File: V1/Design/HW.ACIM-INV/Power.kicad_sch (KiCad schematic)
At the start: 106 parts, among them J1 AC POWER INPUT, J2 FAN, M4 470V/1.2kA, M5 470V/1.2kA, M6 470V/1.2kA, M7 470V/1.2kA, Q10 20V/1A, Q11 20V/1A, U10 SMPS 12V±2%/0.8A, U13 LDO 3.3V±0.5%/1A, U14 SMPS 15V±2%/0.6A, U17 LDO 5V±0.4%/250mA, U20 SMPS 5V±2%/1.2A

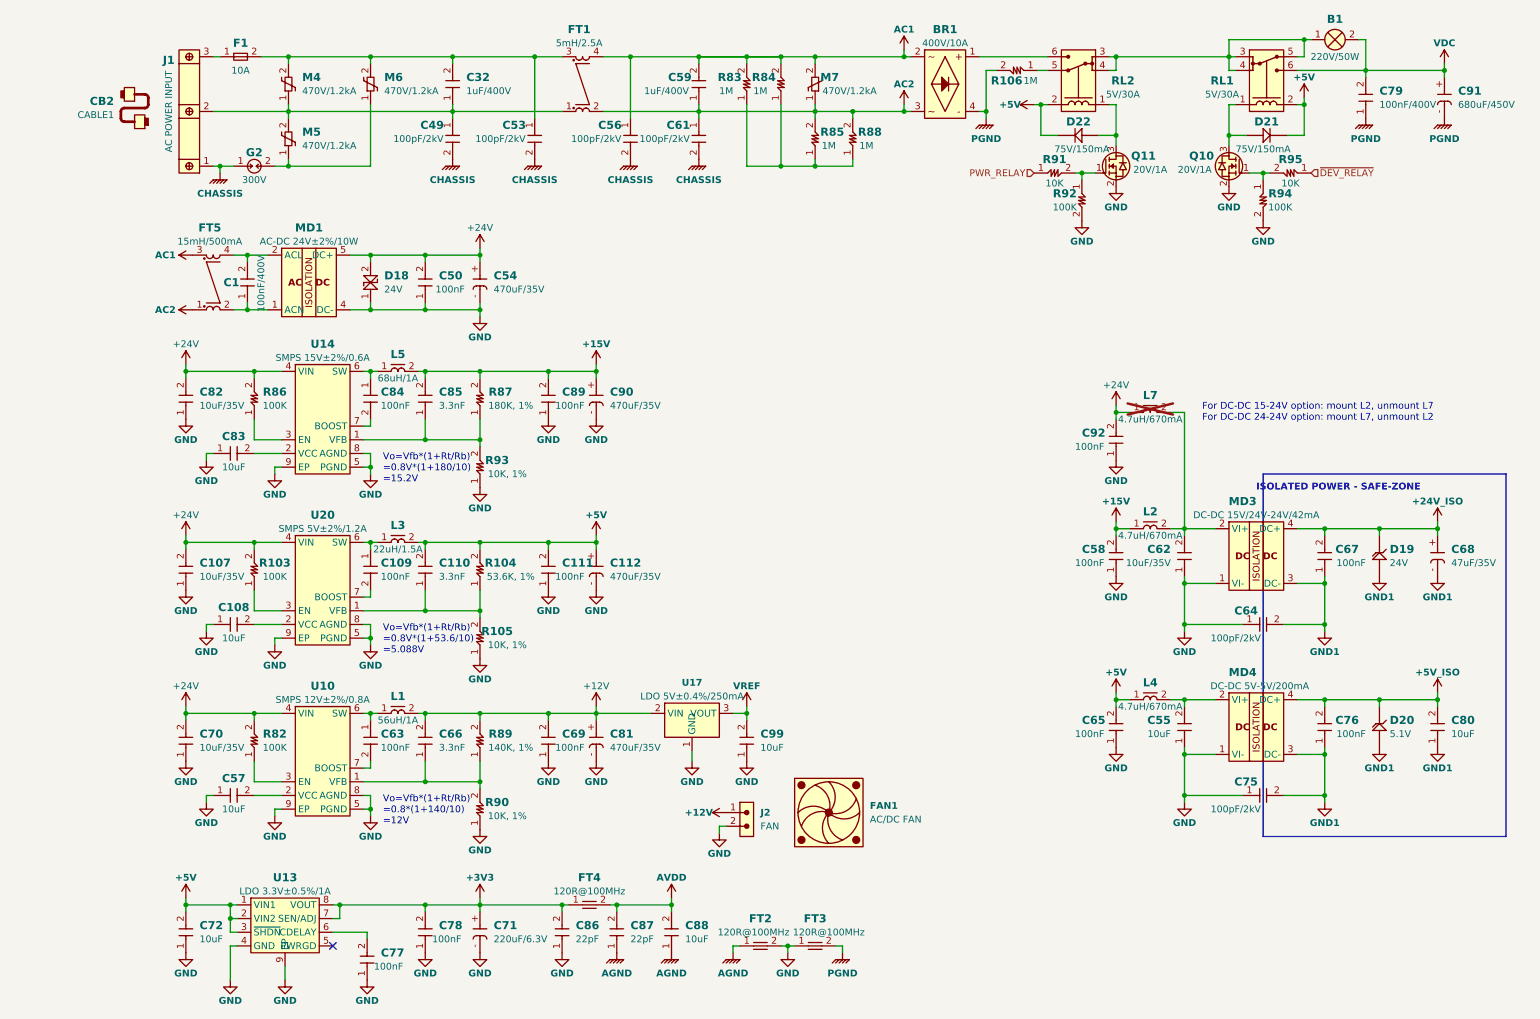
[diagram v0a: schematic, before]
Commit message: V1 schematic update 11
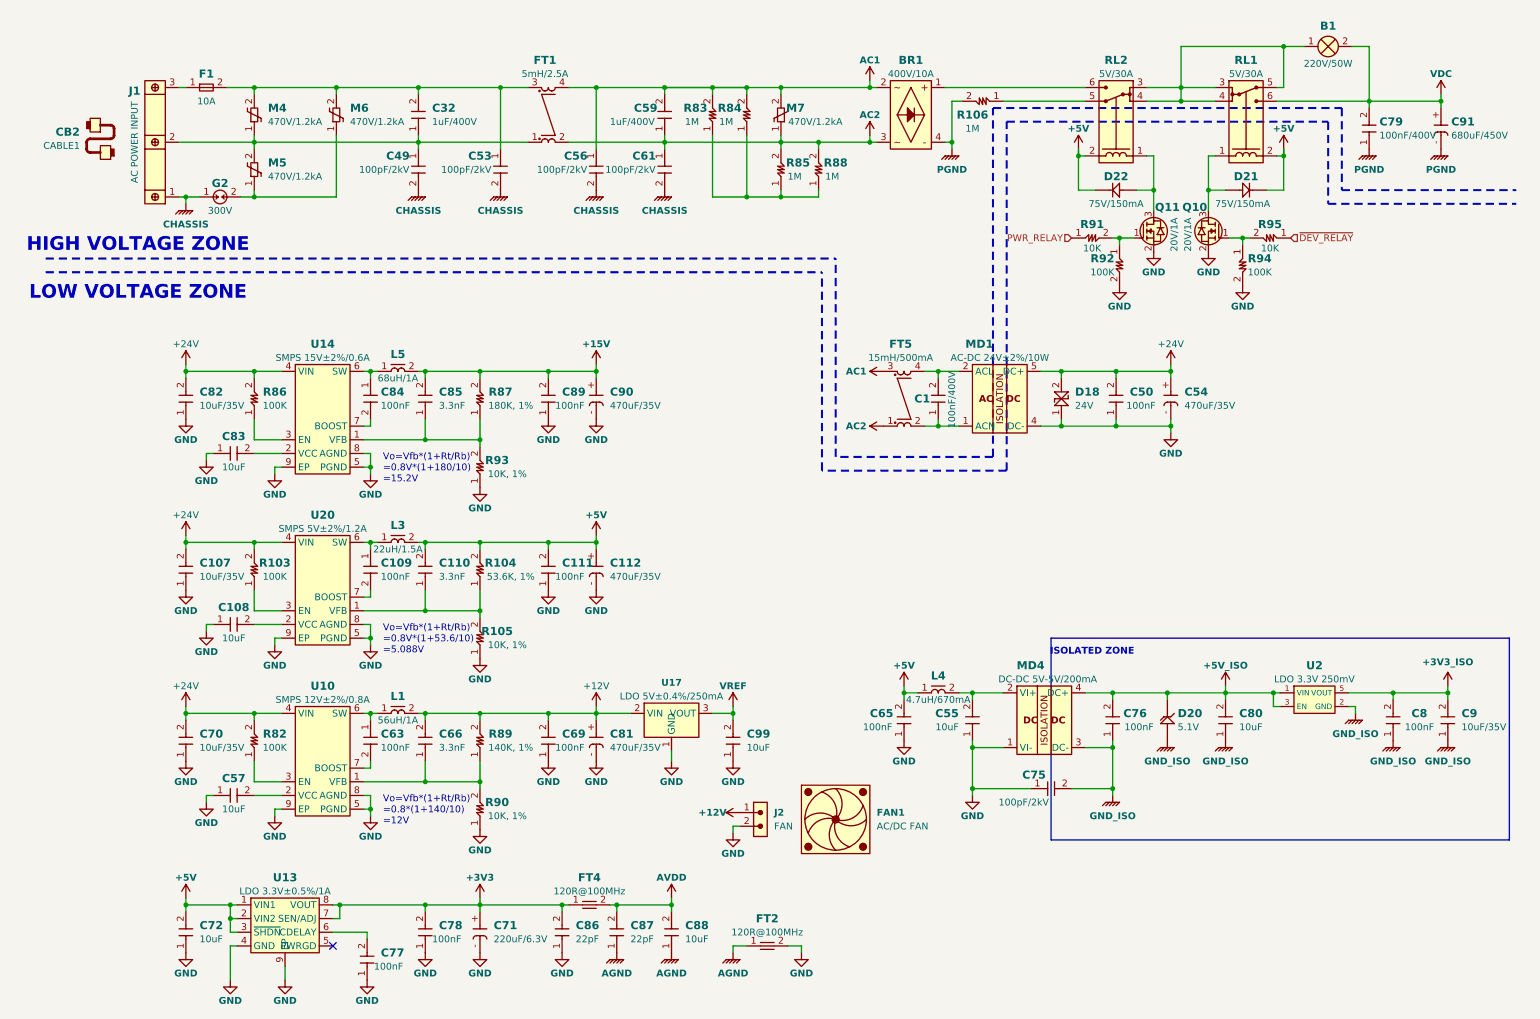
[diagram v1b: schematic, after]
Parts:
- removed C58, C67, C92: 100nF, SAMPI:CAP0603, symbol SAMPI:CERCAP
- removed C62: 10uF/35V, SAMPI:CAP0603, symbol SAMPI:CERCAP
- removed C64: 100pF/2kV, SAMPI:CAP1206, symbol SAMPI:CERCAP
- removed C68: 47uF/35V, SAMPI:CAP_ELEC-6.6x6.6-DIA6.3, symbol SAMPI:ELECCAP
- removed D19: 24V, SAMPI:SOD-80C_DO-213AC, symbol SAMPI:DIODE-ZEN
- removed FT3: 120R@100MHz, SAMPI:FT0603, symbol SAMPI:FerriteBead
- removed L2, L7: 4.7uH/670mA, SAMPI:IND-R5-2MM-TH, symbol SAMPI:IND
- removed MD3: DC-DC 15V/24V-24V/42mA, SAMPI:B1524S-1WR3, symbol SAMPI:DC-DC
- added C8: 100nF, SAMPI:CAP0603, symbol SAMPI:CERCAP
- added C9: 10uF/35V, SAMPI:CAP0603, symbol SAMPI:CERCAP
- added U2: LDO 3.3V 250mV, symbol SAMPI:MIC5504_2
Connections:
- net +5V_ISO: now also U2.1 (VIN), U2.3 (EN)
- net GND1 renamed GND_ISO
- net GND_ISO: now also C8.1, C9.1, U2.2 (GND)
- new net +3V3_ISO: C8.2, C9.2, U2.5 (VOUT)
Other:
- note added: "HIGH VOLTAGE ZONE"
- note added: "ISOLATED ZONE"
- note added: "LOW VOLTAGE ZONE"
- note removed: "For DC-DC 15-24V option: mount L2, unmount L7 For DC-DC 24-24V option: mount L7, unmount L2"
- note removed: "ISOLATED POWER - SAFE-ZONE"
- moved on the sheet: B1, BR1, C1, C32, C49, C50, C53, C54, C55, C56, C59, C61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
